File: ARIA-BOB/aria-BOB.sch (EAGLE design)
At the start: 14 parts

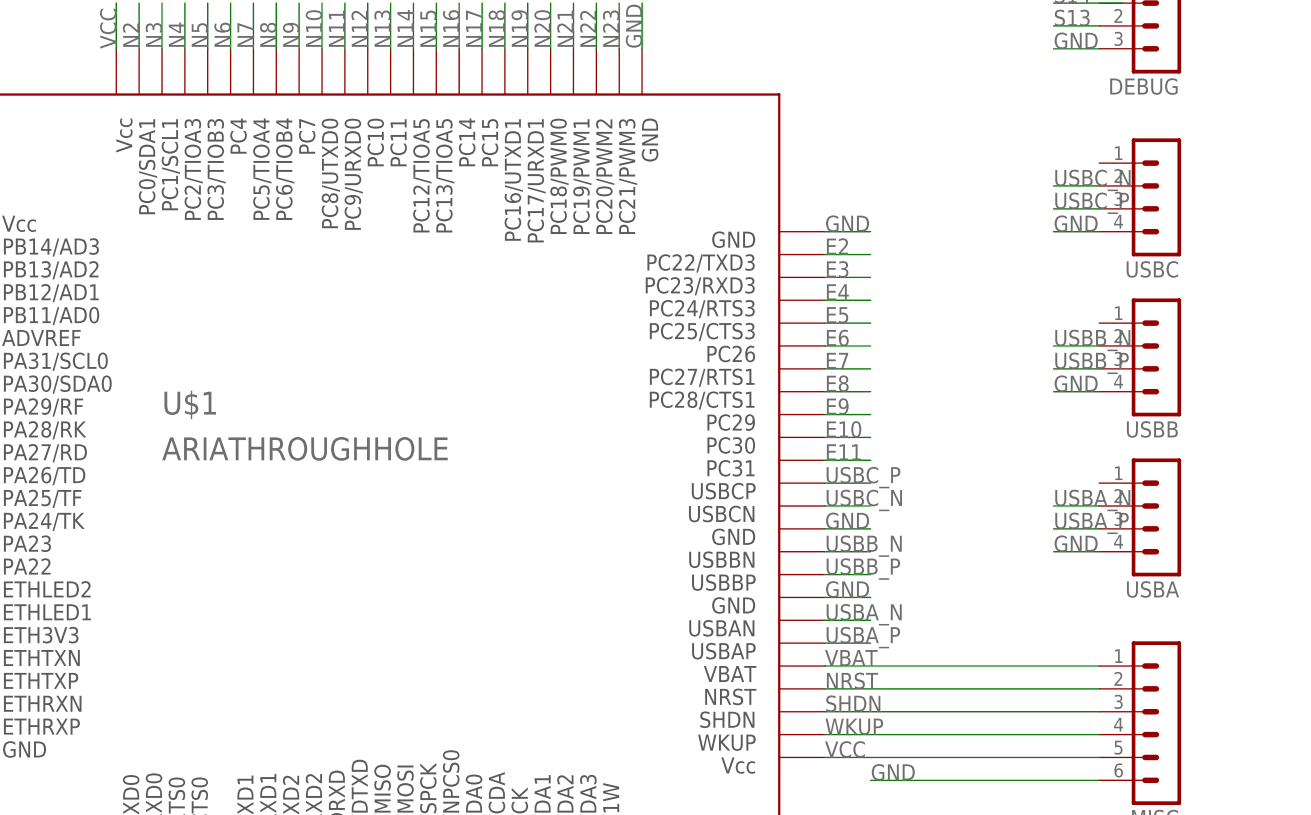
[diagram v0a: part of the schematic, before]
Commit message: revoked changes
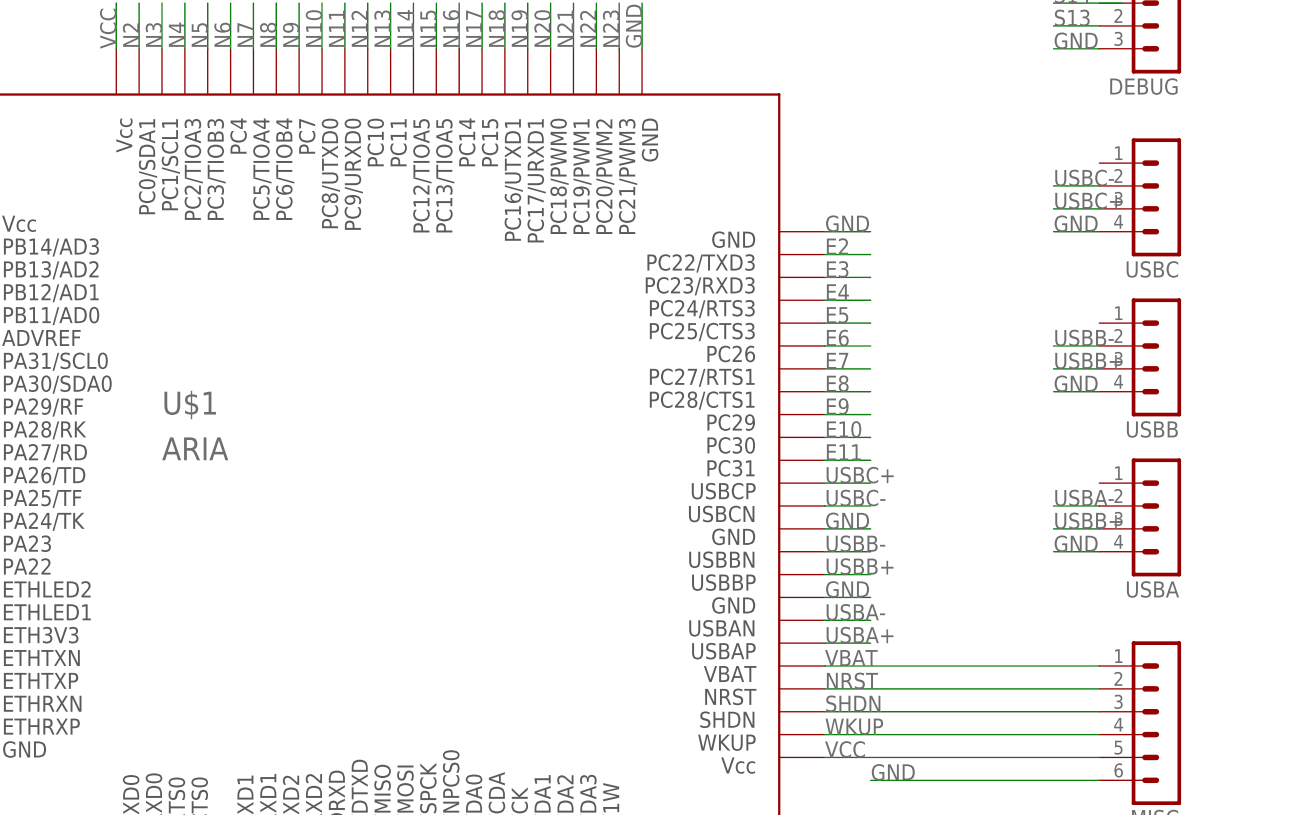
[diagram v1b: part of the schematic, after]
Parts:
- U$1: value ARIATHROUGHHOLE -> ARIA; device octanis-beat:ARIATHROUGHHOLE -> octanis-beat:ARIA
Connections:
- net USBA_N renamed USBA-
- net USBB_N renamed USBB-
- net USBC_N renamed USBC-
- net USBC_P renamed USBC+
- removed net USBA_P: U$1.E19, USBA.3
- removed net USBB_P: U$1.E16, USBB.3
- new net USBA+: U$1.E19
- new net USBB+: U$1.E16, USBA.3, USBB.3
